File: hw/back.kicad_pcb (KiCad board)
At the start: 2 copper layers, 110 x 55 mm, 77 parts, among them J1 IDC_02X13, J2 FC681495, J3 N42GK-04, Q1 BSC080N03MS, U1 OSRB38C9BA, U2 MCP1826S, U3 MCP1826S, U4 BQ24192, U5 LTC1871, U6 LTC2941CMS8E

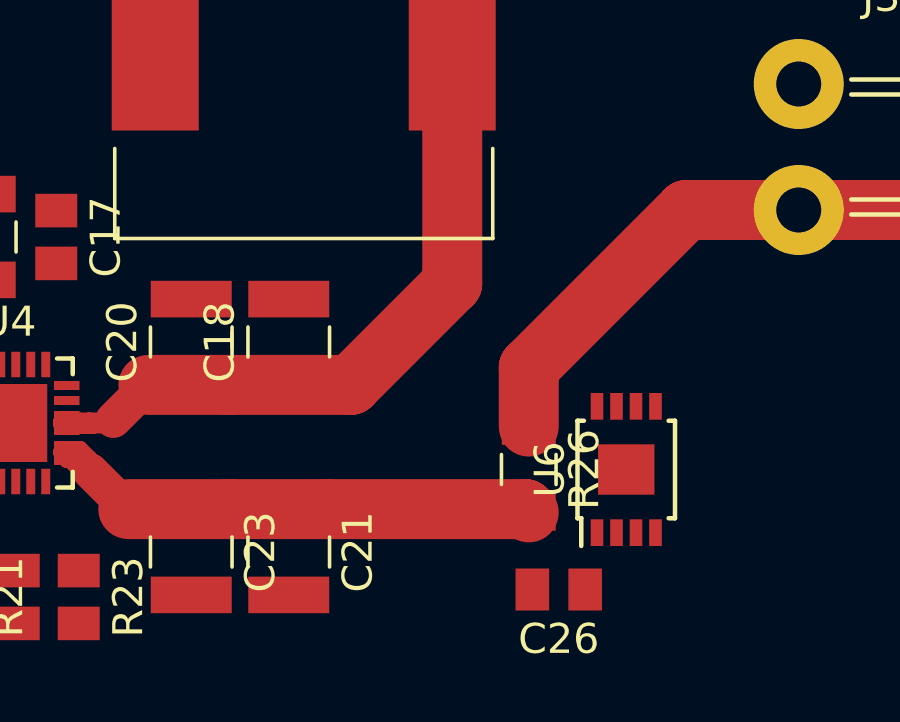
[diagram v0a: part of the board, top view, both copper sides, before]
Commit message: updated pcb
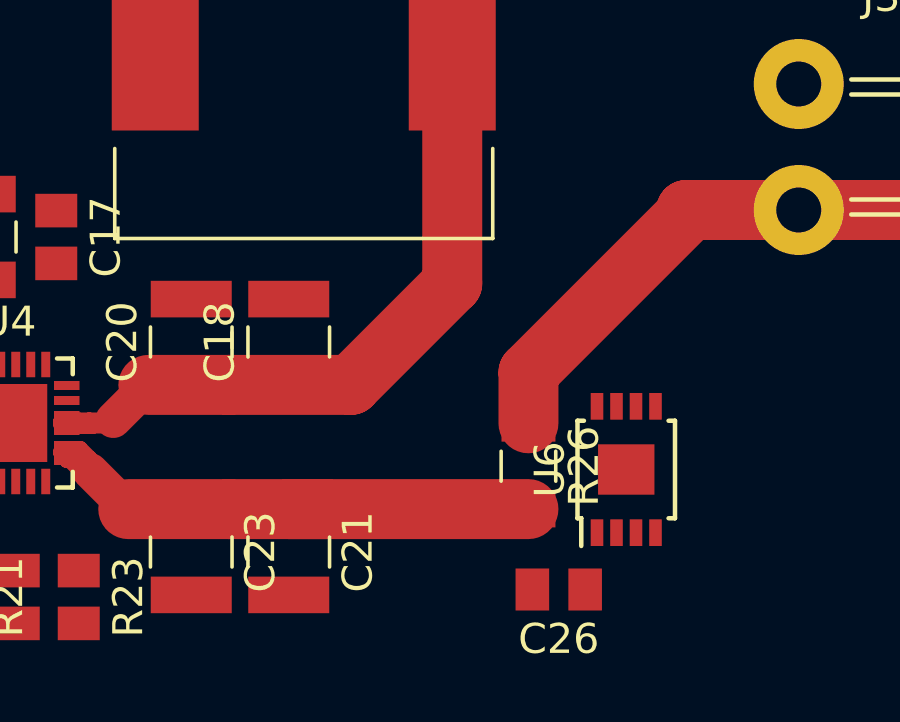
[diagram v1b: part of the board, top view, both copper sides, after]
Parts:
- moved R26 0.11 mm to (159.2, 130.6)
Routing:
- net +BATT: track 79.1 -> 82.3 mm
- net /charger/BAT: track 19.5 -> 20.7 mm
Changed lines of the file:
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@@
     (thickness 1.6)
     (drawings 6)
-    (tracks 125)
+    (tracks 126)
     (zones 0)
     (modules 77)
@@
   )
   (setup
-    (last_trace_width 0.5)
+    (last_trace_width 2)
     (user_trace_width 0.5)
     (user_trace_width 0.8)
@@
   )
   (module Resistor_SMD:R_1206_3216Metric (layer F.Cu)
-    (at 159.25 130.75 270)
+    (at 159.24 130.64 270)
     (descr "Resistor SMD 1206 (3216 Metric), square (rectangular) end terminal, IPC_7351 nominal, (Body size source: http://www.tortai-tech.com/upload/download/2011102023233369053.pdf), generated with kicad-footprint-generator")
     (tags resistor)
@@
   (gr_line (start 200 85) (end 200 140) (layer Edge.Cuts) (width 0.15))
   (gr_line (start 90 85) (end 200 85) (layer Edge.Cuts) (width 0.15))
-  (segment (start 159.25 129.32) (end 159.25 127.35) (width 2) (layer F.Cu) (net 1))
-  (segment (start 159.25 127.35) (end 164.5 122.1) (width 2) (layer F.Cu) (net 1))
+  (segment (start 159.24 129.21) (end 159.24 127.51) (width 2) (layer F.Cu) (net 1))
+  (segment (start 159.24 127.51) (end 164.5 122.25) (width 2) (layer F.Cu) (net 1))
+  (segment (start 164.5 122.25) (end 164.5 122.1) (width 2) (layer F.Cu) (net 1))
   (segment (start 164.5 122.1) (end 168.25 122.1) (width 2) (layer F.Cu) (net 1))
   (segment (start 173.75 122.1) (end 168.25 122.1) (width 2) (layer F.Cu) (net 1))
+  (segment (start 151.25 132.07) (end 159.24 132.07) (width 2) (layer F.Cu) (net 2))
   (segment (start 144.299999 130.050001) (end 144.630001 130.380003) (width 0.5) (layer F.Cu) (net 2))
   (segment (start 144.630001 130.380003) (end 144.630001 130.800001) (width 0.5) (layer F.Cu) (net 2))
@@
   (segment (start 145.9 132.07) (end 144.630001 130.800001) (width 1.2) (layer F.Cu) (net 2))
   (segment (start 149.25 132.07) (end 145.9 132.07) (width 2) (layer F.Cu) (net 2))
-  (segment (start 152.5 132.07) (end 159.14 132.07) (width 2) (layer F.Cu) (net 2))
-  (segment (start 159.14 132.07) (end 159.25 132.18) (width 2) (layer F.Cu) (net 2))
   (segment (start 149.25 132.07) (end 152.5 132.07) (width 2) (layer F.Cu) (net 2))
   (segment (start 111.62 91) (end 111.62 88.46) (width 2) (layer F.Cu) (net 3))
@@
   (segment (start 132.5 94.36) (end 131.94 93.8) (width 0.5) (layer F.Cu) (net 29))
   (segment (start 132.5 96.37) (end 132.5 94.36) (width 0.5) (layer F.Cu) (net 29))
+  (segment (start 148 127.93) (end 151.25 127.93) (width 0.5) (layer F.Cu) (net 31))
   (segment (start 144.15 129.3) (end 145.2 129.3) (width 0.5) (layer F.Cu) (net 31))
   (segment (start 145.2 129.3) (end 145.4 129.1) (width 0.5) (layer F.Cu) (net 31))
